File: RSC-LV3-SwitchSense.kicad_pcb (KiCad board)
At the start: 2 copper layers, 140 x 85 mm, 183 parts, among them J1 FTSH-105-01-L-DV-K-A, J10 Molex 43045-0400, J11 Molex 43045-0400, J12 Molex 43045-0400, J13 Molex 43045-0400, J14 Molex 43045-0400, J15 Molex 43045-0400, J16 Molex 43650-0200, J2 USB_C_Receptacle_USB2.0_16P, J3 Molex 43650-0500, J4 Molex 43650-0500, J5 Molex 43650-0200, J6 Molex 43045-0400, J7 Molex 43045-0400, J8 Molex 43045-0400, J9 Molex 43045-0400, Q1 AO3400A, Q10 AO3400A, Q2 AO3400A, Q3 AO3400A, Q4 AO3400A, Q5 AO3400A, Q6 AO3400A, Q7 AO3400A, Q8 AO3400A, Q9 AO3400A, U1 STM32G0B1CBTx, U2 TPS54302, U3 TLV74033PDBVR, U4 TJA1051T-3, U5 TJA1051T-3, Y1 Crystal_GND24, Y2 32.768 kHz 6pF

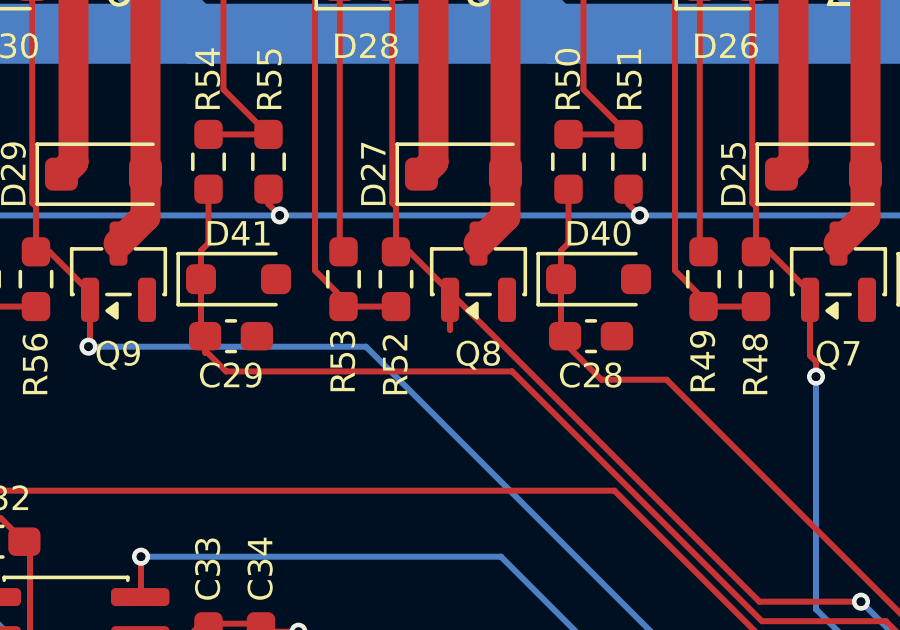
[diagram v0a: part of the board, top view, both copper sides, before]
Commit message: minor layout and silkscreen changes
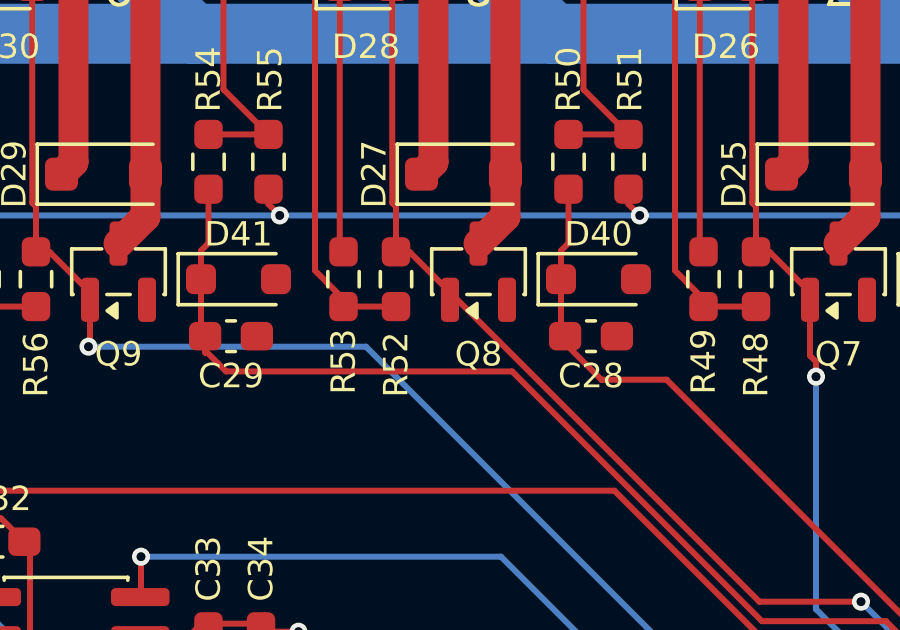
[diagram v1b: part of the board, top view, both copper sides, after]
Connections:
- J2 pad SH: (no net) -> GND
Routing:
- net OUT_8: track 48.3 -> 47.3 mm
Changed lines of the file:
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@@
 			(layers "*.Cu" "*.Mask")
 			(remove_unused_layers no)
+			(net "GND")
 		)
 		(pad "SH" thru_hole oval
@@
 			(layers "*.Cu" "*.Mask")
 			(remove_unused_layers no)
+			(net "GND")
 		)
 		(pad "SH" thru_hole oval
@@
 			(layers "*.Cu" "*.Mask")
 			(remove_unused_layers no)
+			(net "GND")
 		)
 		(pad "SH" thru_hole oval
@@
 			(layers "*.Cu" "*.Mask")
 			(remove_unused_layers no)
+			(net "GND")
 		)
 		(embedded_fonts no)
@@
 		)
 	)
+	(barcode
+		(at 91.5 113.5 0)
+		(layer "B.SilkS")
+		(size 15 15)
+		(text "https://cy2.me/pcb/rsc-lv3-switchsense-r0")
+		(text_height 1)
+		(type qr)
+		(ecc_level M)
+		(hide yes)
+		(knockout no)
+	)
 	(dimension
 		(type orthogonal)
@@
 		(width 0.2)
 		(layer "F.Cu")
-		(net "OUT_8")
-	)
-	(segment
-		(start 109.05 75.1875)
-		(end 109.05 76.2)
-		(width 0.2)
-		(layer "F.Cu")
